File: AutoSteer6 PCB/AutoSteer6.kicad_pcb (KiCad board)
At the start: 2 copper layers, 100 x 100 mm, 41 parts, among them J1 SDA, J10 Power In, J2 SCL, J3 I2C-5V, J4 Steering, J5 Power Source, J6 VCC, J7 Roll/Pitch, J8 Motor Control, J9 Motor Power, U1 ADS1115

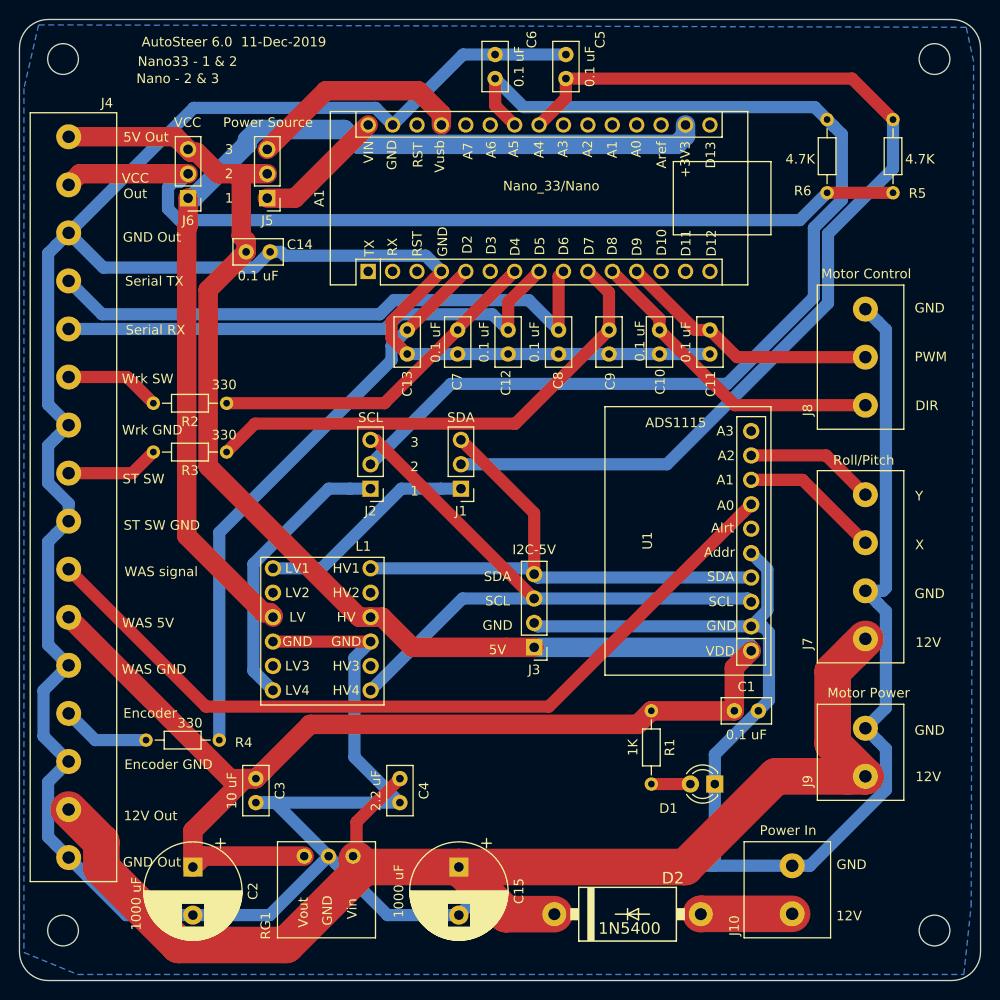
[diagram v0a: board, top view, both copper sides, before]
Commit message: update pcb
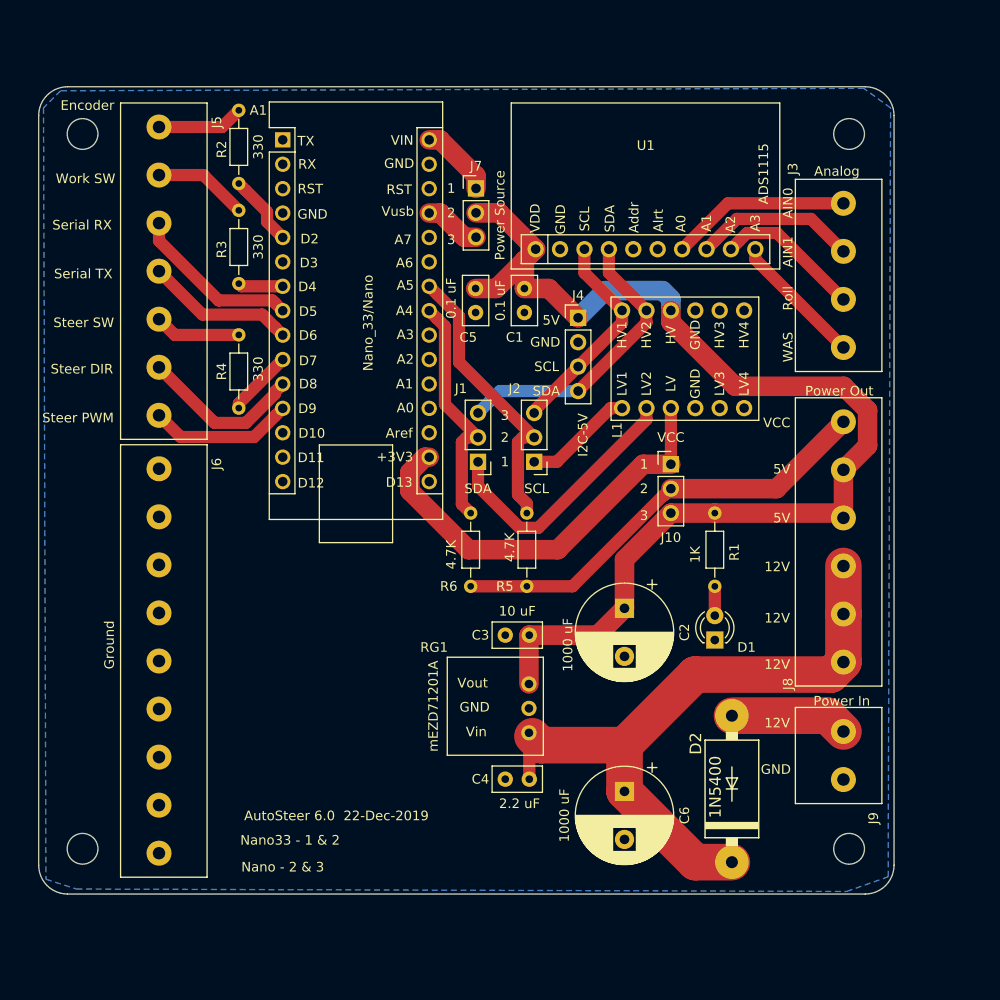
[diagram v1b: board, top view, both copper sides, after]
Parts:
- removed C10, C11, C12, C13, C7, C8, C9: 0.1 uF, Capacitor_THT:C_Disc_D5.0mm_W2.5mm_P2.50mm
- removed the C5 at (133.9, 57.1)
- removed the C6 at (126.5, 57.1)
- removed the J4 at (87.1, 60.7)
- removed the J7 at (160.0, 117.9)
- removed the J9 at (160.0, 132.3)
- added J3: Analog, my library:Phoenix_4_pin_5mm_terminal_block, F.Cu at (157.7, 87.6)
- added J5: GPIO's, my library:Phoenix_7_pin_5mm_terminal_block, F.Cu at (96.5, 59.7)
- added J6: Ground, my library:Phoenix_9_pin_5mm_terminal_block, F.Cu at (96.5, 95.2)
- J8: value Motor Control -> Power Out; footprint my library:Phoenix_3_pin_5mm_terminal_block -> my library:Phoenix_6_pin_5mm_terminal_block
- moved R2 65.6 mm to (99.8, 60.5), turned to 270 degrees
- moved L1 62.7 mm to (157.5, 78.7), turned to 90 degrees
- moved R6 60.1 mm to (124.0, 110.0)
- moved J10 57.4 mm to (144.8, 97.3), turned to 0 degrees
- moved C2 52.4 mm to (140.0, 112.3)
- moved R5 51.5 mm to (129.8, 110.0)
- moved U1 49.1 mm to (129.0, 76.5), turned to 0 degrees
- moved C1 49.1 mm to (129.5, 79.0), turned to 270 degrees
- moved J4 34.6 mm to (135.1, 82.0), turned to 0 degrees
- moved C3 32.1 mm to (130.0, 115.1), turned to 180 degrees
- moved J8 26.8 mm to (157.7, 120.4)
- moved C5 24.2 mm to (124.5, 79.0), turned to 270 degrees
- moved J7 21.7 mm to (124.5, 68.6), turned to 0 degrees
- moved R1 21.6 mm to (149.4, 102.4)
- moved RG1 20.4 mm to (121.5, 127.6), turned to 90 degrees
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- renumbered C14 to C5, C15 to C6, J6 to J10, J3 to J4, J5 to J7, J10 to J9, R4 to R2, R2 to R3, R3 to R4, R6 to R5, R5 to R6
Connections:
- C4 pad 1: Net-(C15-Pad1) -> Net-(C4-Pad1)
- C6 pad 1: Net-(C15-Pad1) -> Net-(C4-Pad1)
- D2 pad C: Net-(C15-Pad1) -> Net-(C4-Pad1)
- J10 pad 2: Net-(J4-Pad2) -> Net-(J10-Pad2)
- J8 pad 1: Net-(A1-Pad26) -> Net-(C4-Pad1)
- J8 pad 2: Net-(A1-Pad27) -> Net-(C4-Pad1)
- J8 pad 3: GND -> Net-(C4-Pad1)
- J9 pad 1: Net-(D2-PadA) -> GND
- J9 pad 2: GND -> Net-(D2-PadA)
- L1 pad 1: Net-(J1-Pad1) -> Net-(J2-Pad1)
- L1 pad 12: Net-(J2-Pad3) -> Net-(L1-Pad12)
- L1 pad 2: Net-(L1-Pad2) -> Net-(J1-Pad1)
- L1 pad 6: Net-(J2-Pad1) -> Net-(L1-Pad6)
- L1 pad 7: Net-(J1-Pad3) -> Net-(J2-Pad3)
- L1 pad 8: Net-(L1-Pad8) -> Net-(J1-Pad3)
- R2 pad 1: Net-(A1-Pad20) -> Net-(J5-Pad1)
- R2 pad 2: Net-(J4-Pad13) -> Net-(A1-Pad20)
- R3 pad 1: Net-(A1-Pad22) -> Net-(J5-Pad2)
- R3 pad 2: Net-(J4-Pad6) -> Net-(A1-Pad22)
- R4 pad 1: Net-(A1-Pad25) -> Net-(J5-Pad5)
- R4 pad 2: Net-(J4-Pad8) -> Net-(A1-Pad25)
- R5 pad 1: Net-(J4-Pad2) -> Net-(J10-Pad2)
- R6 pad 1: Net-(J4-Pad2) -> Net-(J10-Pad2)
- RG1 pad 1: Net-(C15-Pad1) -> Net-(C4-Pad1)
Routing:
- net GND: track 490.6 -> 0.00 mm
- net Net-(C15-Pad1): track 138.0 -> 0.00 mm
- net Net-(C1-Pad1): track 229.7 -> 121.8 mm
- net Net-(J4-Pad2): track 94.9 -> 0.00 mm
- net Net-(A1-Pad9): track 115.6 -> 29.9 mm
- net Net-(A1-Pad8): track 108.8 -> 24.9 mm
- net Net-(C4-Pad1): track 0.00 -> 70.2 mm
- net Net-(J3-Pad4): track 85.7 -> 18.8 mm
- net Net-(A1-Pad2): track 104.9 -> 43.8 mm
- net Net-(A1-Pad20): track 59.4 -> 7.51 mm
- net Net-(J10-Pad2): track 0.00 -> 45.9 mm
- net Net-(J2-Pad3): track 67.6 -> 22.5 mm
- net Net-(A1-Pad25): track 52.1 -> 6.95 mm
- net Net-(A1-Pad24): track 60.6 -> 15.6 mm
- net Net-(A1-Pad23): track 54.5 -> 17.7 mm
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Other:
- board size 100 x 100 mm -> 89 x 84 mm
- board text added: "AIN0"
- board text added: "AIN1"
- board text added: "AutoSteer 6.0 22-Dec-2019"
- board text added: "Roll"
- board text added: "Steer DIR"
- board text added: "Steer PWM"
- board text added: "Steer SW"
- board text added: "VCC"
- board text added: "WAS"
- board text added: "Work SW"
- board text removed: "12V Out"
- board text removed: "5V Out"
- board text removed: "AutoSteer 6.0 11-Dec-2019"
- board text removed: "DIR"
- board text removed: "Encoder GND"
- board text removed: "GND Out"
- board text removed: "PWM"
- board text removed: "ST SW"
- board text removed: "ST SW GND"
- board text removed: "VCC Out"
- board text removed: "WAS 5V"
- board text removed: "WAS GND"
- board text removed: "WAS signal"
- board text removed: "Wrk GND"
- board text removed: "Wrk SW"
- board text removed: "X"
- board text removed: "Y"
